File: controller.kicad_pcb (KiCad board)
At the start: 2 copper layers, 156.8 x 70.7 mm, 56 parts, among them J1 Conn_ST_STDC14, J2 USB_C_Receptacle_USB2.0_14P, SW1 SW_Push, SW10 SW_Push, SW11 SW_Push, SW12 SW_Push, SW13 SW_Push, SW2 SW_Push, SW3 SW_Push, SW4 SW_Push, SW5 SW_Push, SW6 SW_Push, SW8 SW_Push, SW9 SW_Push, U1 STM32L476RGTx, U2 BD33FC0FP, U3 NUP2202

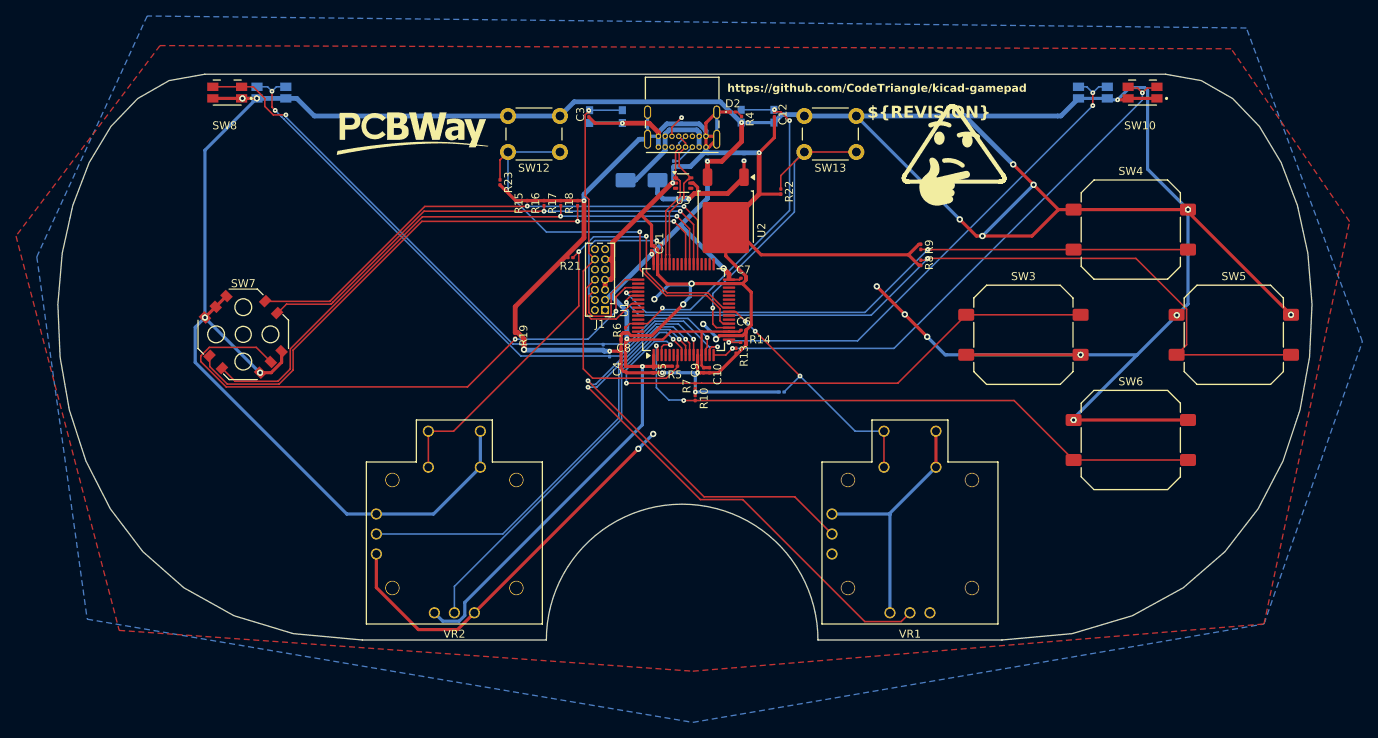
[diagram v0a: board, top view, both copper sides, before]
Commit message: final commit before i do something really silly
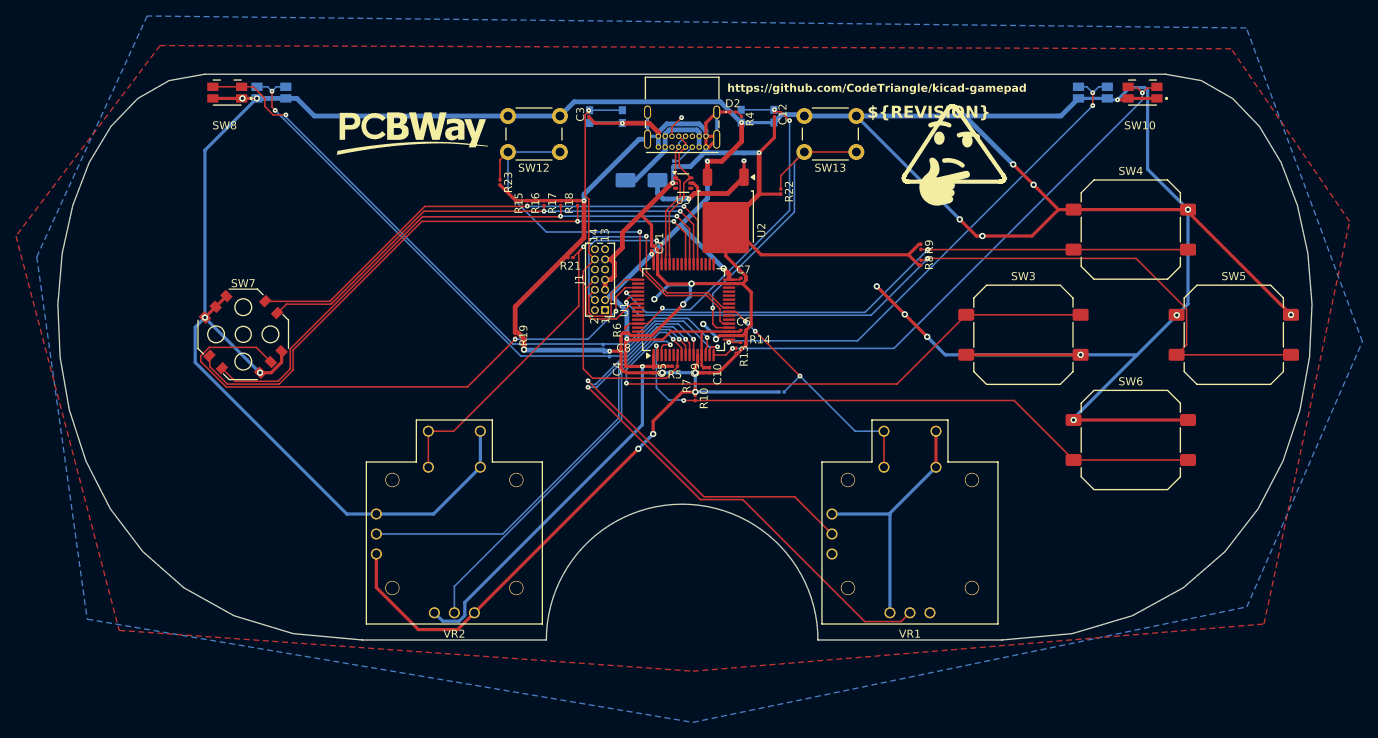
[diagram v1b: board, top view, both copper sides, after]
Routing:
- net +3.3V: track 601.0 -> 592.0 mm
- net GND: track 327.7 -> 336.6 mm
- net LeftClick: track 63.5 -> 64.4 mm
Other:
- board text added: "1"
- board text added: "13"
- board text added: "14"
- board text added: "2"
